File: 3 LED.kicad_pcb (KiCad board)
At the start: 2 copper layers, 24 x 48 mm, 14 parts, among them J1 Conn_01x04_Socket, Q1 NPN, Q2 NPN, Q3 NPN, U1 74HC238

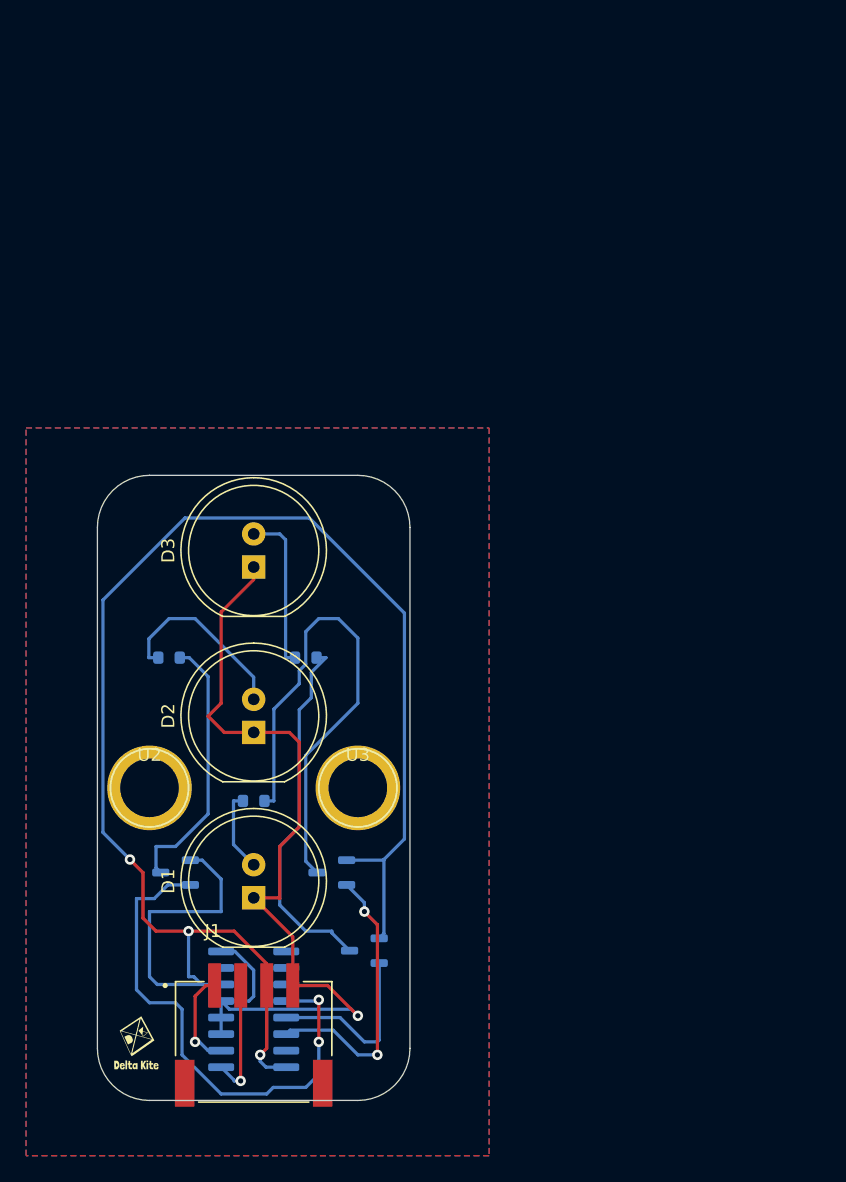
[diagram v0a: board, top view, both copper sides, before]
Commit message: On Production
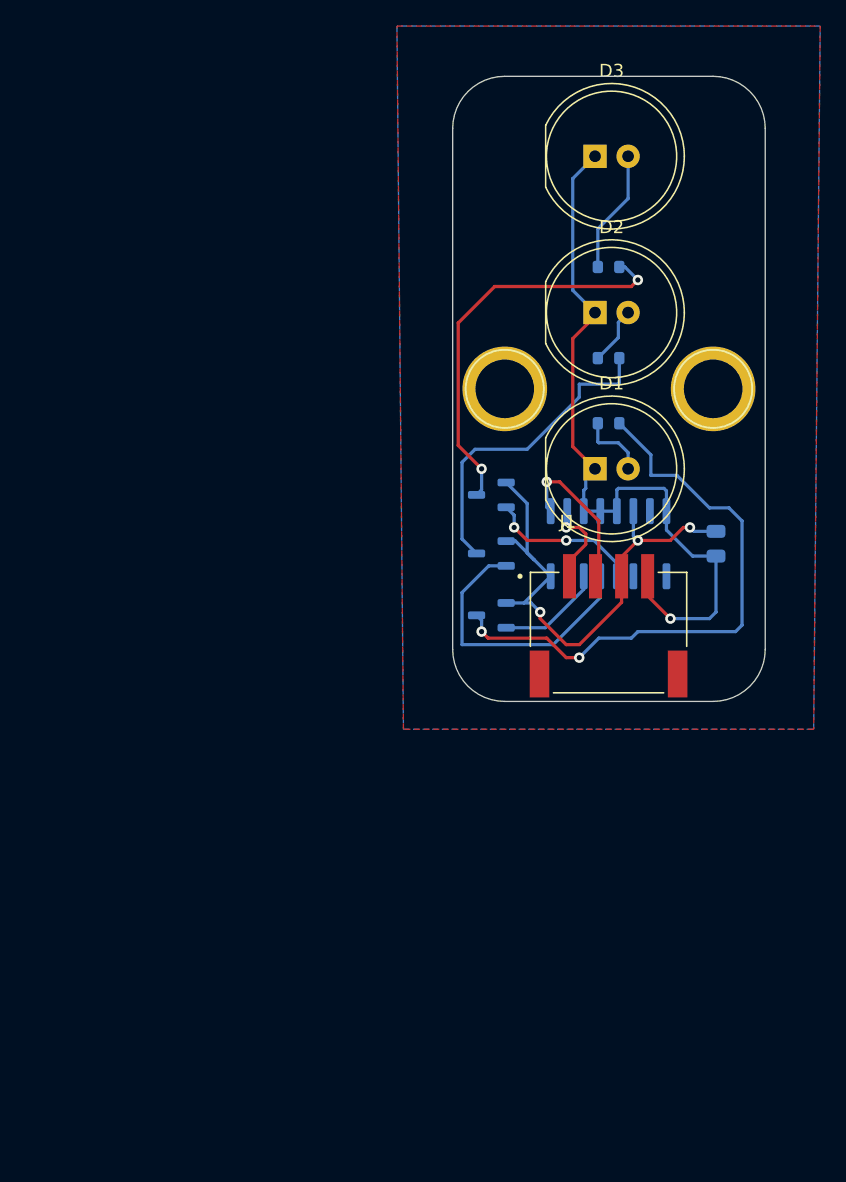
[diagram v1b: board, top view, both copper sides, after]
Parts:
- removed the G*** at (105.0, 133.5)
- removed U2, U3: ~, Library_Custom:LEGO HOLE 4.5-6.5
- added C1: C, Capacitor_SMD:C_0805_2012Metric, B.Cu at (149.5, 95.2)
- added G***: LOGO, DeltaKiteEngineering:BKU_Medium, B.Cu at (148.0, 72.5)
- added G***: LOGO, DeltaKiteEngineering:DeltaKite_Large, B.Cu at (148.0, 65.0)
- added REF**: Module Base, Library_Custom:Module Base, F.Cu at (142.2, 111.8)
- moved R3 45.2 mm to (141.2, 74.0)
- moved U1 45.0 mm to (141.2, 95.2), turned to -90 degrees
- moved D1 42.1 mm to (140.2, 89.5), turned to 0 degrees
- moved J1 41.6 mm to (141.2, 102.1)
- moved D2 41.5 mm to (140.2, 77.5), turned to 0 degrees
- moved D3 41.0 mm to (140.2, 65.5), turned to 0 degrees
- moved R1 39.8 mm to (141.2, 86.0)
- moved Q3 37.8 mm to (132.2, 91.5)
- moved R2 32.7 mm to (141.2, 81.0)
- moved Q2 32.0 mm to (132.2, 96.0)
- moved Q1 23.2 mm to (132.2, 100.8)
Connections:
- R2 pad 2: Net-(D3-A) -> Net-(D2-A)
- R3 pad 2: Net-(D2-A) -> Net-(D3-A)
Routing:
- net +5V: track 130.4 -> 40.3 mm
- net /L3: track 39.8 -> 11.8 mm
- net /L1: track 21.9 -> 8.18 mm, vias 2 -> 0
- net GND: track 70.6 -> 58.2 mm
- net Net-(Q3-E): track 20.5 -> 31.1 mm, vias 0 -> 2
- net Net-(D2-A): track 14.4 -> 4.46 mm
- net /L2: track 13.9 -> 22.0 mm
- net Net-(Q1-E): track 39.8 -> 44.7 mm, vias 0 -> 2
- net Net-(Q2-E): track 28.1 -> 24.6 mm
- net Net-(D3-A): track 12.4 -> 9.46 mm
- net /S0: track 9.29 -> 12.0 mm
- net Net-(D1-A): track 6.27 -> 5.34 mm
- net /S1: track 7.62 -> 6.76 mm

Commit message: Production Version
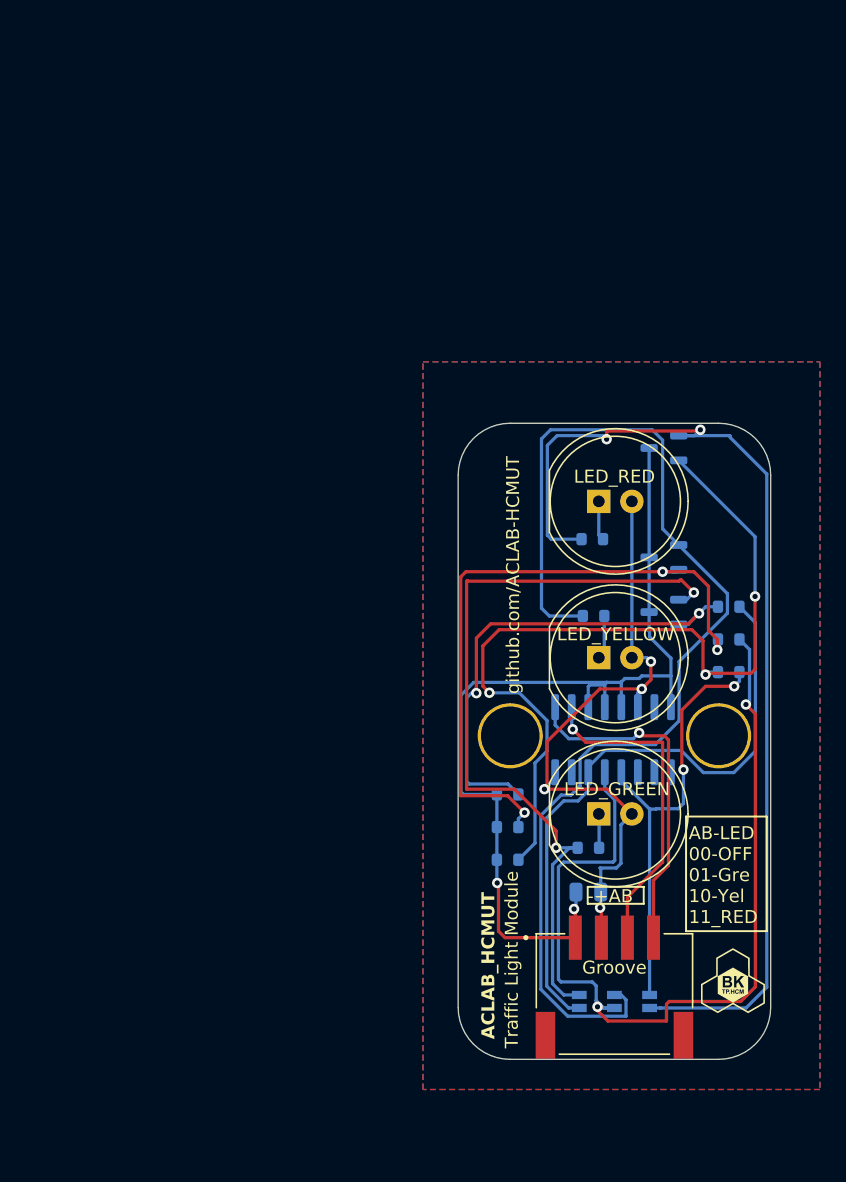
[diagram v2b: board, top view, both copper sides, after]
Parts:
- removed D1, D2, D3: LED, LED_THT:LED_D10.0mm
- removed the G*** at (148.0, 65.0)
- removed J1: Conn_01x04_Socket, Library_Custom:SEEEDSTUDIO_114020164
- removed the REF** at (142.2, 111.8)
- added Groove: Conn_01x04_Socket, Library_Custom:SEEEDSTUDIO_114020164, F.Cu at (141.7, 129.8)
- added JP1: Jumper_2_Open, SofleRGB:Jumper, B.Cu at (139.0, 130.4)
- added JP2: Jumper_2_Open, SofleRGB:Jumper, B.Cu at (141.7, 130.4)
- added JP3: Jumper_2_Open, SofleRGB:Jumper, B.Cu at (144.4, 130.4)
- added LED_GREEN: LED, LED_THT:LED_D10.0mm, F.Cu at (140.5, 116.0)
- added LED_RED: LED, LED_THT:LED_D10.0mm, F.Cu at (140.5, 92.0)
- added LED_YELLOW: LED, LED_THT:LED_D10.0mm, F.Cu at (140.5, 104.0)
- added R4: R, Resistor_SMD:R_0603_1608Metric, B.Cu at (150.5, 100.1)
- added R5: R, Resistor_SMD:R_0603_1608Metric, B.Cu at (150.5, 102.6)
- added R6: R, Resistor_SMD:R_0603_1608Metric, B.Cu at (150.5, 105.1)
- added R7: R, Resistor_SMD:R_0603_1608Metric, B.Cu at (133.5, 114.5)
- added R8: R, Resistor_SMD:R_0603_1608Metric, B.Cu at (133.5, 117.0)
- added R9: R, Resistor_SMD:R_0603_1608Metric, B.Cu at (133.5, 119.5)
- added REF**: Ohstem_Base, ACLAB:Ohstem_Base_V2, F.Cu at (142.6, 116.1)
- G***: moved to F.Cu
- U1: value 74HC238 -> 74HC238D
- moved G*** 56.4 mm to (150.8, 128.8), turned to 0 degrees
- moved R1 32.6 mm to (139.7, 118.6)
- moved C1 28.5 mm to (139.7, 122.0), turned to 180 degrees
- moved R3 20.9 mm to (140.0, 94.9)
- moved R2 19.8 mm to (140.1, 100.8)
- moved U1 15.1 mm to (141.6, 110.3)
- moved Q3 13.7 mm to (145.5, 87.9)
- moved Q2 13.3 mm to (145.5, 96.3)
- moved Q1 13.3 mm to (145.5, 100.5)
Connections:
- Q1 pad 1: +5V -> Net-(JP1-A)
- Q1 pad 2: /L1 -> Net-(Q1-B)
- Q1 pad 3: Net-(Q1-E) -> GND
- Q2 pad 1: +5V -> Net-(JP2-A)
- Q2 pad 2: /L2 -> Net-(Q2-B)
- Q2 pad 3: Net-(Q2-E) -> GND
- Q3 pad 1: +5V -> Net-(JP3-B)
- Q3 pad 2: /L3 -> Net-(Q3-B)
- Q3 pad 3: Net-(Q3-E) -> GND
- R1 pad 1: Net-(Q1-E) -> Net-(D1-K)
- R1 pad 2: Net-(D1-A) -> Net-(JP1-A)
- R2 pad 1: Net-(Q2-E) -> Net-(D2-K)
- R2 pad 2: Net-(D2-A) -> Net-(JP2-A)
- R3 pad 1: Net-(Q3-E) -> Net-(D3-K)
- R3 pad 2: Net-(D3-A) -> Net-(JP3-B)
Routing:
- net Net-(JP2-A): track 0.00 -> 89.4 mm
- net Net-(JP3-B): track 0.00 -> 81.5 mm, vias 0 -> 2
- net Net-(Q3-B): track 0.00 -> 64.7 mm, vias 0 -> 3
- net Net-(JP1-A): track 0.00 -> 60.4 mm, vias 0 -> 2
- net Net-(Q2-B): track 0.00 -> 50.5 mm, vias 0 -> 3
- net /L2: track 22.0 -> 70.0 mm, vias 0 -> 2
- net Net-(Q1-E): track 44.7 -> 0.00 mm, vias 2 -> 0
- net /L1: track 8.18 -> 48.3 mm
- net Net-(Q1-B): track 0.00 -> 37.8 mm, vias 0 -> 2
- net Net-(Q3-E): track 31.1 -> 0.00 mm, vias 2 -> 0
- net Net-(Q2-E): track 24.6 -> 0.00 mm
- net /L3: track 11.8 -> 34.0 mm
- net /S1: track 6.76 -> 25.2 mm
- net GND: track 58.2 -> 74.9 mm, vias 1 -> 2
- net /S0: track 12.0 -> 26.7 mm
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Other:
- board size 24 x 48 mm -> 24 x 48.8 mm
- board text added: "-+AB"
- board text added: "AB-LED 00-OFF 01-Gre 10-Yel 11_RED"
- board text added: "ACLAB_HCMUT"
- board text added: "Traffic Light Module"
- board text added: "github.com/ACLAB-HCMUT"
